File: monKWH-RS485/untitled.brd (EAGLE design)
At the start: 77 x 60 mm, 49 parts, among them J1 U.FL-R-SMT(01), J2 DCJ0202, J3 10103594, Q1 MMBT3904, Q2 MMBT3904, Q3 12MHz, U1 RT9193-33GB, U2 RT9193-33GB, X1 MSTBA2, X2 MSTBA2

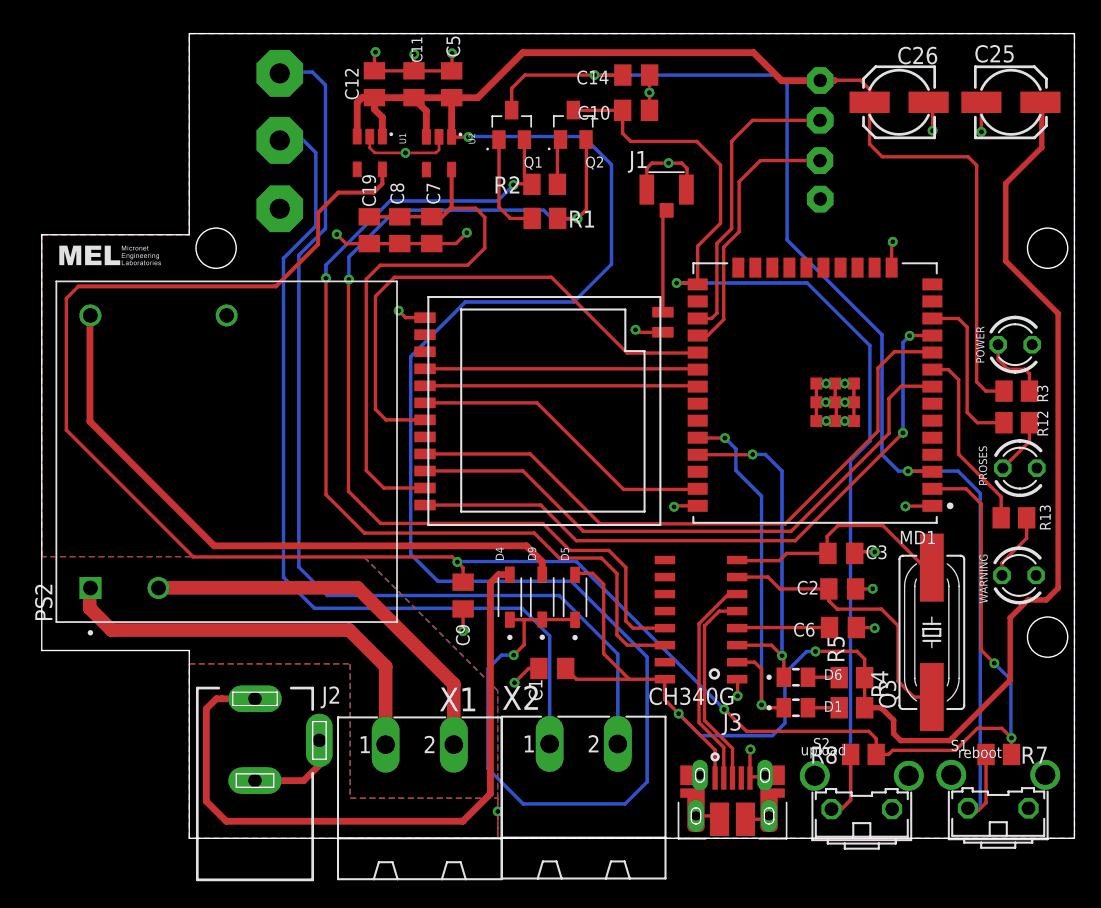
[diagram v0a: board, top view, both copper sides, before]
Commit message: PCBv1.0
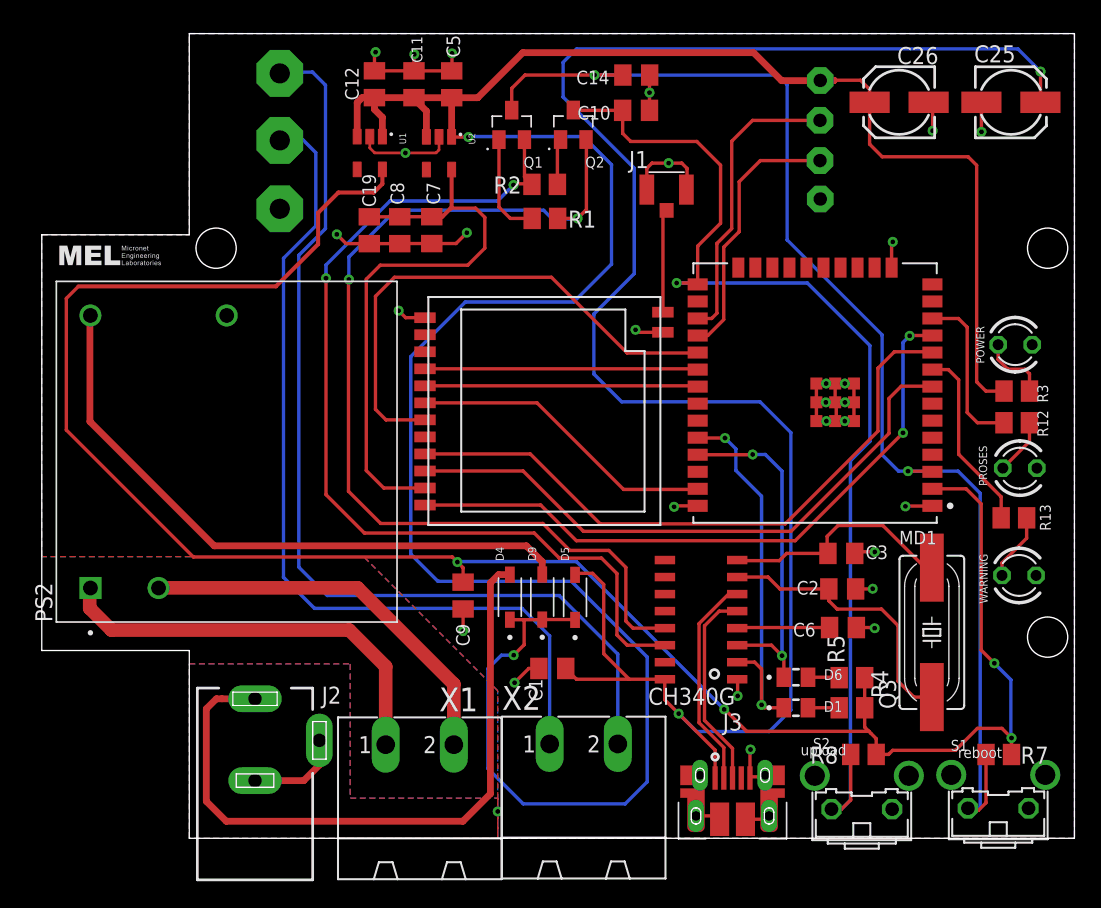
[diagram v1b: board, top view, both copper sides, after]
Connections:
- net 3V3: now also R4.2, R5.2
- net VCC: no longer R4.2, R5.2
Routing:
- net VCC: track 112.7 -> 139.8 mm
- net 3V3: track 147.1 -> 151.2 mm
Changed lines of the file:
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@@
 <drawing>
 <settings>
-<setting alwaysvectorfont="yes"/>
+<setting alwaysvectorfont="no"/>
 <setting verticaltext="up"/>
 </settings>
-<grid distance="1" unitdist="mm" unit="mm" style="lines" multiple="1" display="yes" altdistance="5" altunitdist="mil" altunit="mm"/>
+<grid distance="0.003125" unitdist="mic" unit="mm" style="lines" multiple="1" display="yes" altdistance="5" altunitdist="mil" altunit="mm"/>
 <layers>
 <layer number="1" name="Top" color="4" fill="1" visible="yes" active="yes"/>
@@
 <wire x1="75.262740625" y1="51.816" x2="75.262740625" y2="47.5259375" width="0.254" layer="16"/>
 <wire x1="65.218059375" y1="46.25390625" x2="65.218059375" y2="47.4284" width="0.254" layer="1"/>
-<wire x1="65.218059375" y1="47.4284" x2="64.670940625" y2="47.97551875" width="0.254" layer="1"/>
+<wire x1="65.218059375" y1="47.4284" x2="64.823228125" y2="47.82323125" width="0.254" layer="1"/>
+<wire x1="64.823228125" y1="47.82323125" x2="64.670940625" y2="47.97551875" width="0.254" layer="1"/>
 <wire x1="64.670940625" y1="47.97551875" x2="55.557421875" y2="47.97551875" width="0.254" layer="1"/>
 <wire x1="55.557421875" y1="47.97551875" x2="53.90388125" y2="49.629059375" width="0.254" layer="1"/>
@@
 <via x="33.989009375" y="60.598053125" extent="1-16" drill="0.35"/>
 <wire x1="42.8625" y1="60.632340625" x2="34.023296875" y2="60.632340625" width="0.254" layer="16"/>
+<contactref element="R4" pad="2"/>
+<contactref element="R5" pad="2"/>
+<wire x1="64.360653125" y1="49.730953125" x2="64.360665625" y2="49.730965625" width="0.254" layer="1"/>
+<wire x1="64.360653125" y1="51.974965625" x2="64.360653125" y2="50" width="0.254" layer="1"/>
+<wire x1="64.360653125" y1="50" x2="64.360653125" y2="49.730978125" width="0.254" layer="1"/>
+<wire x1="64.360653125" y1="49.730978125" x2="64.360665625" y2="49.730965625" width="0.254" layer="1"/>
+<wire x1="64.670940625" y1="47.97551875" x2="64.360653125" y2="48.28580625" width="0.254" layer="1"/>
+<wire x1="64.360653125" y1="48.28580625" x2="64.360653125" y2="49.730978125" width="0.254" layer="1"/>
 </signal>
 <signal name="N$12">
@@
 </signal>
 <signal name="VCC">
-<contactref element="R4" pad="2"/>
-<contactref element="R5" pad="2"/>
 <contactref element="C1" pad="1"/>
 <contactref element="U$2" pad="16"/>
@@
 <contactref element="C25" pad="+"/>
 <contactref element="J3" pad="1"/>
-<wire x1="64.360653125" y1="49.730953125" x2="64.360665625" y2="49.730965625" width="0.254" layer="1"/>
 <wire x1="42.06919375" y1="52.662759375" x2="42.8741" y2="51.857853125" width="0.254" layer="1"/>
 <wire x1="46.805909375" y1="51.857853125" x2="42.8741" y2="51.857853125" width="0.254" layer="1"/>
@@
 <wire x1="44.07408125" y1="59.756040625" x2="42.8746875" y2="59.756040625" width="0.254" layer="1"/>
 <wire x1="42.8746875" y1="59.756040625" x2="42.763678125" y2="59.64503125" width="0.254" layer="1"/>
-<wire x1="64.360653125" y1="51.974965625" x2="64.360653125" y2="49.730978125" width="0.254" layer="1"/>
-<wire x1="64.360653125" y1="49.730978125" x2="64.360665625" y2="49.730965625" width="0.254" layer="1"/>
 <wire x1="53.206115625" y1="44.4947125" x2="53.206115625" y2="46.577784375" width="0.254" layer="1"/>
 <wire x1="49.4538" y1="50.3301" x2="49.4538" y2="51.857853125" width="0.254" layer="1"/>
 <wire x1="53.206115625" y1="46.577784375" x2="50.49011875" y2="49.29378125" width="0.254" layer="1"/>
 <wire x1="50.49011875" y1="49.29378125" x2="49.4538" y2="50.3301" width="0.254" layer="1"/>
-<wire x1="64.360665625" y1="49.730965625" x2="65.590115625" y2="49.730965625" width="0.4064" layer="1"/>
-<wire x1="65.590115625" y1="49.730965625" x2="66.5226" y2="48.79848125" width="0.4064" layer="1"/>
-<wire x1="66.5226" y1="48.79848125" x2="66.5226" y2="47.800259375" width="0.4064" layer="1"/>
-<wire x1="66.5226" y1="47.800259375" x2="67.040759375" y2="47.2821" width="0.4064" layer="1"/>
-<wire x1="67.040759375" y1="47.2821" x2="70.698359375" y2="47.2821" width="0.4064" layer="1"/>
-<wire x1="70.698359375" y1="47.2821" x2="75.209396875" y2="51.7931375" width="0.4064" layer="1"/>
-<wire x1="75.209396875" y1="51.7931375" x2="75.209396875" y2="56.441340625" width="0.4064" layer="1"/>
-<wire x1="75.209396875" y1="56.441340625" x2="76.53805625" y2="57.77" width="0.4064" layer="1"/>
-<wire x1="77.899659375" y1="57.77" x2="78.7808" y2="58.651140625" width="0.4064" layer="1"/>
-<wire x1="76.53805625" y1="57.77" x2="77.899659375" y2="57.77" width="0.4064" layer="1"/>
-<wire x1="78.7808" y1="58.651140625" x2="78.7808" y2="79.128459375" width="0.4064" layer="1"/>
-<wire x1="78.7808" y1="79.128459375" x2="74.881740625" y2="83.02751875" width="0.4064" layer="1"/>
-<wire x1="74.881740625" y1="83.02751875" x2="74.881740625" y2="88.826340625" width="0.4064" layer="1"/>
-<wire x1="74.881740625" y1="88.826340625" x2="77.56398125" y2="91.50858125" width="0.4064" layer="1"/>
-<wire x1="77.56398125" y1="91.50858125" x2="77.56398125" y2="94.77539375" width="0.4064" layer="1"/>
 <wire x1="77.56398125" y1="94.77539375" x2="77.462690625" y2="94.876684375" width="0.4064" layer="1"/>
-<wire x1="64.360653125" y1="51.974965625" x2="64.360653125" y2="53.360728125" width="0.254" layer="1"/>
-<wire x1="64.360653125" y1="53.360728125" x2="63.7794" y2="53.94198125" width="0.254" layer="1"/>
-<wire x1="63.7794" y1="53.94198125" x2="60.708540625" y2="53.94198125" width="0.254" layer="1"/>
-<wire x1="60.708540625" y1="53.94198125" x2="60.6933" y2="53.926740625" width="0.254" layer="1"/>
-<via x="60.6933" y="53.926740625" extent="1-16" drill="0.35"/>
-<wire x1="60.6933" y1="53.926740625" x2="60.03798125" y2="53.926740625" width="0.254" layer="16"/>
-<wire x1="60.03798125" y1="53.926740625" x2="58.4073" y2="52.296059375" width="0.254" layer="16"/>
-<wire x1="58.4073" y1="52.296059375" x2="58.4073" y2="48.56988125" width="0.254" layer="16"/>
-<wire x1="58.4073" y1="48.56988125" x2="57.4929" y2="47.65548125" width="0.254" layer="16"/>
-<wire x1="57.4929" y1="47.65548125" x2="52.113178125" y2="47.65548125" width="0.254" layer="16"/>
-<wire x1="52.113178125" y1="47.65548125" x2="50.4825" y2="49.286159375" width="0.254" layer="16"/>
 <wire x1="50.4825" y1="49.286159375" x2="50.4825" y2="49.2861625" width="0.254" layer="16"/>
 <wire x1="50.4825" y1="49.2861625" x2="50.49011875" y2="49.29378125" width="0.254" layer="16"/>
 <via x="50.49011875" y="49.29378125" extent="1-16" drill="0.35"/>
+<wire x1="50.49011875" y1="49.29378125" x2="51.82206875" y2="47.96183125" width="0.254" layer="16"/>
+<wire x1="58.853625" y1="49.5670625" x2="58.853625" y2="70.249734375" width="0.254" layer="16"/>
+<wire x1="58.853625" y1="70.249734375" x2="56.558365625" y2="72.54499375" width="0.254" layer="16"/>
+<wire x1="56.558365625" y1="72.54499375" x2="46.239290625" y2="72.54499375" width="0.254" layer="16"/>
+<wire x1="46.239290625" y1="72.54499375" x2="44.173321875" y2="74.6109625" width="0.254" layer="16"/>
+<wire x1="44.173321875" y1="74.6109625" x2="44.173321875" y2="79.099678125" width="0.254" layer="16"/>
+<wire x1="44.173321875" y1="79.099678125" x2="47.18111875" y2="82.107475" width="0.254" layer="16"/>
+<wire x1="47.18111875" y1="82.107475" x2="47.18111875" y2="89.962765625" width="0.254" layer="16"/>
+<wire x1="47.18111875" y1="89.962765625" x2="41.873240625" y2="95.27064375" width="0.254" layer="16"/>
+<wire x1="41.873240625" y1="95.27064375" x2="41.873240625" y2="97.8544" width="0.254" layer="16"/>
+<wire x1="41.873240625" y1="97.8544" x2="42.875840625" y2="98.857" width="0.254" layer="16"/>
+<wire x1="42.875840625" y1="98.857" x2="75.7856625" y2="98.857" width="0.254" layer="16"/>
+<wire x1="75.7856625" y1="98.857" x2="77.473240625" y2="97.169421875" width="0.254" layer="16"/>
+<via x="77.473240625" y="97.169421875" extent="1-16" drill="0.35"/>
+<wire x1="77.473240625" y1="97.169421875" x2="77.473240625" y2="94.866134375" width="0.254" layer="1"/>
+<wire x1="77.473240625" y1="94.866134375" x2="77.56398125" y2="94.77539375" width="0.254" layer="1"/>
+<wire x1="51.82206875" y1="47.96183125" x2="57.24839375" y2="47.96183125" width="0.254" layer="16"/>
+<wire x1="57.24839375" y1="47.96183125" x2="58.853625" y2="49.5670625" width="0.254" layer="16"/>
 </signal>
 <signal name="N$3">
